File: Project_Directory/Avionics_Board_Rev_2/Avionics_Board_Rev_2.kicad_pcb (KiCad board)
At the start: 2 copper layers, 60 x 130 mm, 86 parts, among them J1 Battery, J10 PWM_1, J11 PWM_2, J12 PWM_3, J13 I2C, J14 UART, J15 Conn_Coaxial, J16 ON, J2 ARM, J3 PYRO_1, J4 PYRO_3, J5 PYRO_2, J6 PYRO_4, J7 PWM_4, J8 PWM_5, J9 PWM_6, Q1 Drive_MOS, Q2 Drive_MOS, Q3 Drive_MOS, Q4 Drive_MOS, Q5 Drive_MOS, SW1 SW_DPDT_x2, U1 Teensy4.1, U10 GSM, U11 AP2127K-3.3, U2 LoRa - RFM95-W/PW, U3 ADXL, U4 ADS1115IDGS, U5 AMS1117-3.3, U6 GPS, U7 GY-91, U8 AMS1117-5.0

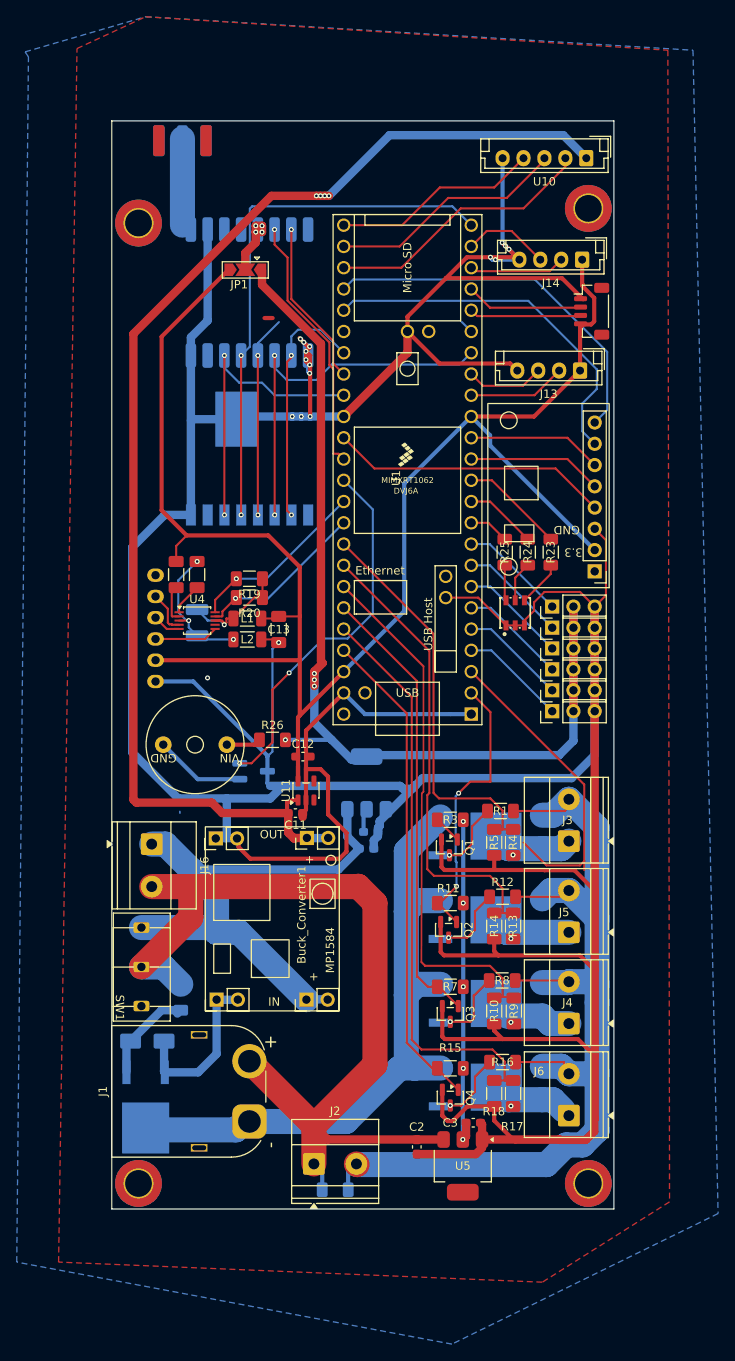
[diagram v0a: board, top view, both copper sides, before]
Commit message: modification 1 7 mmarch
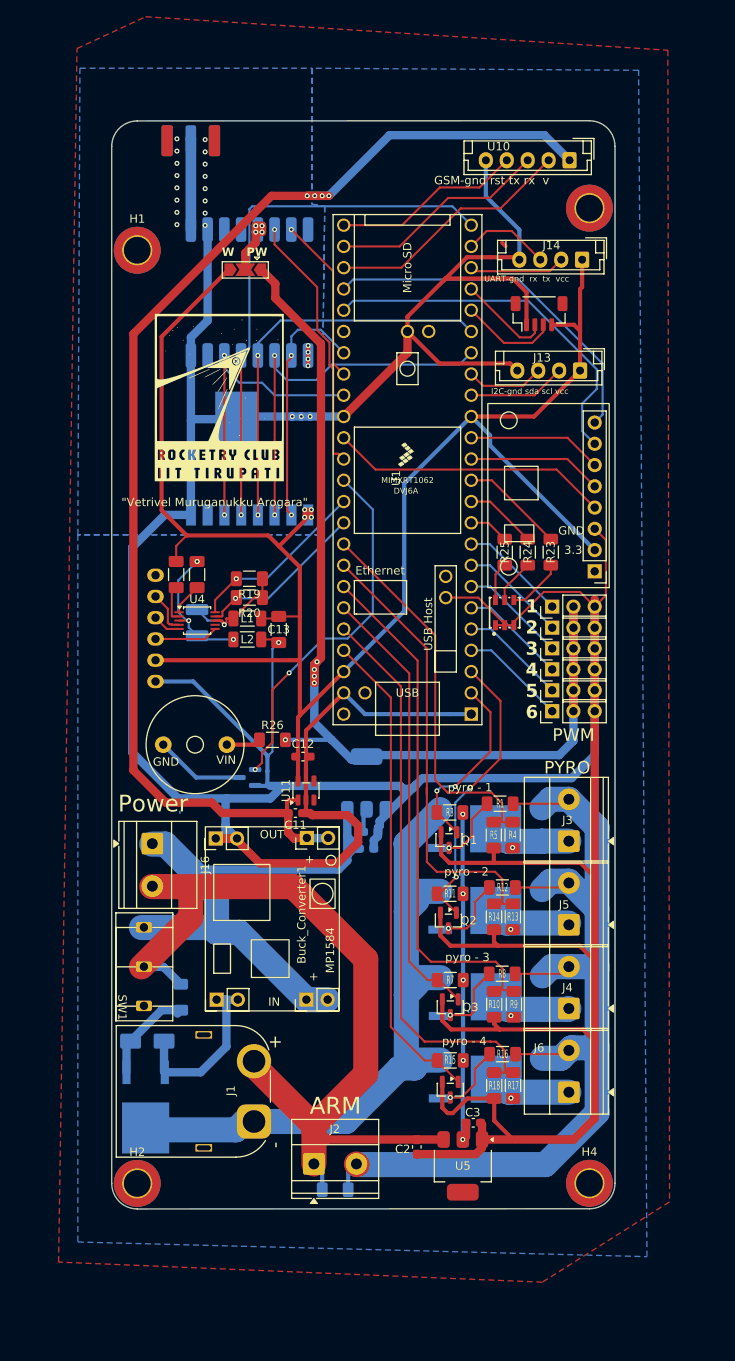
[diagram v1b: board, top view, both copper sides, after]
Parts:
- removed REF** (x4): MountingHole_3.2mm_M3_DIN965_Pad_TopBottom, MountingHole:MountingHole_3.2mm_M3_DIN965_Pad_TopBottom
- added G***: LOGO, VelR:VelR logo 1.5_2cm, F.Cu at (135.6, 58.3)
- added H1: MountingHole_Pad, MountingHole:MountingHole_3.2mm_M3_DIN965_Pad_TopBottom, F.Cu at (125.8, 40.7)
- added H2: MountingHole_Pad, MountingHole:MountingHole_3.2mm_M3_DIN965_Pad_TopBottom, F.Cu at (125.8, 152.2)
- added H3: MountingHole_Pad, MountingHole:MountingHole_3.2mm_M3_DIN965_Pad_TopBottom, F.Cu at (179.8, 35.7)
- added H4: MountingHole_Pad, MountingHole:MountingHole_3.2mm_M3_DIN965_Pad_TopBottom, F.Cu at (179.8, 152.2)
- Q5: footprint Package_TO_SOT_SMD:SC-59_Handsoldering -> Package_TO_SOT_SMD:SOT-23
- moved U6 6.38 mm to (174.0, 48.0), turned to 0 degrees
- moved J6 2.80 mm to (177.4, 141.3)
- moved U10 2.02 mm to (177.4, 29.9)
- moved J4 1.80 mm to (177.4, 131.3)
- moved LED1 1.26 mm to (169.7, 84.0)
- moved C9 1.11 mm to (166.1, 119.6)
- moved D4 1.11 mm to (174.2, 119.1)
- moved Q2 1.11 mm to (163.0, 120.8)
- moved R11 1.11 mm to (163.2, 117.6)
- moved R12 1.11 mm to (169.4, 116.8)
- moved R13 1.11 mm to (170.7, 120.3)
- moved R14 1.11 mm to (168.4, 120.3)
- moved Q5 1.06 mm to (138.9, 103.7), turned to 180 degrees
- moved J15 1.00 mm to (132.2, 27.4)
- moved C10 0.95 mm to (166.2, 139.8)
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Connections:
- Q5 pad 1: Net-(BZ1-GND) -> /Buzzer
- Q5 pad 2: /Buzzer -> GND
- Q5 pad 3: GND -> Net-(BZ1-GND)
- U1 pad 2: /PYRO_2_Trig -> /PYRO_1_Trig
- U1 pad 3: /PYRO_1_Trig -> /PYRO_2_Trig
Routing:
- net /PYRO_3_continuity: track 28.4 -> 62.9 mm
- net /SPI1_SCK: track 25.7 -> 47.7 mm
- net GND: track 600.7 -> 579.0 mm, vias 17 -> 24
- net /PYRO_1_Trig: track 41.3 -> 22.3 mm, vias 0 -> 2
- net +3.3V: track 201.1 -> 211.8 mm, vias 0 -> 4
- net +BATT: track 109.9 -> 104.1 mm
- net +BATT_C: track 67.0 -> 72.1 mm
- net +VDC: track 128.6 -> 124.1 mm
- net +5V: track 129.7 -> 132.8 mm, vias 4 -> 5
- net /GPS_RX: track 14.3 -> 11.2 mm
- net /GSM_RX: track 32.5 -> 30.0 mm
- net /GSM_TX: track 28.5 -> 26.2 mm
- net /GSM_RST: track 24.8 -> 22.7 mm
- net /GPS_TX: track 13.7 -> 11.6 mm
- net /BUCK_Out: track 151.5 -> 149.7 mm
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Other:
- board size 60 x 130 mm -> 60.1 x 130 mm
- board text added: "1 2 3 4 5 6"
- board text added: "ARM"
- board text added: "GSM-gnd rst tx rx v"
- board text added: "I2C-gnd sda scl vcc"
- board text added: "PWM"
- board text added: "PYRO"
- board text added: "Power"
- board text added: "UART-gnd rx tx vcc"
- board text added: "W PW"
- board text added: "put kapton tape on for isolation"
- board text added: "pyro - 1"
- board text added: "pyro - 2"
- board text added: "pyro - 3"
- board text added: "pyro - 4"
- board text added: "{dblquote}Vetrivel Muruganukku Arogara{dblquote}"
